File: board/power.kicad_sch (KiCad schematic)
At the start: 16 parts, among them J2 768250002, U2 OKI-78SR-12_1.0-W36H-C, U3 SHHD003A0A

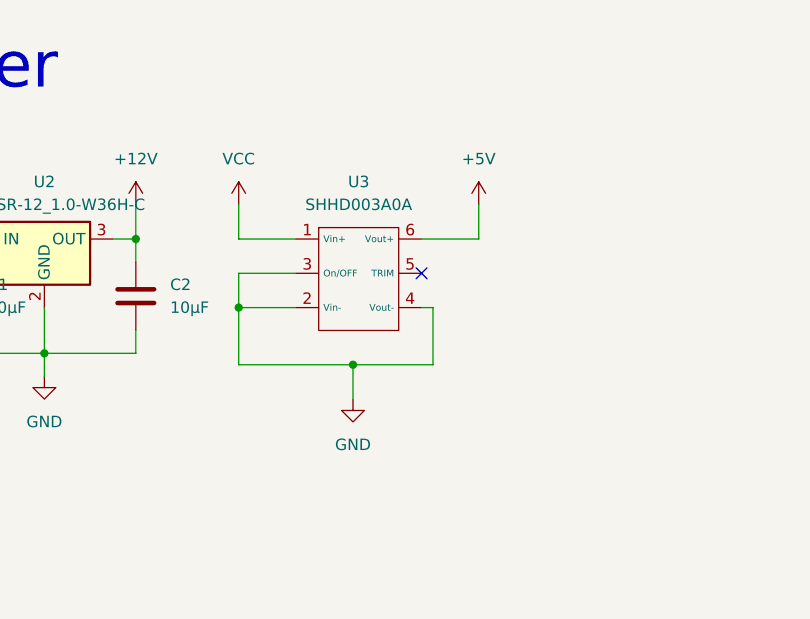
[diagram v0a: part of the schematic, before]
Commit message: rev2 progress
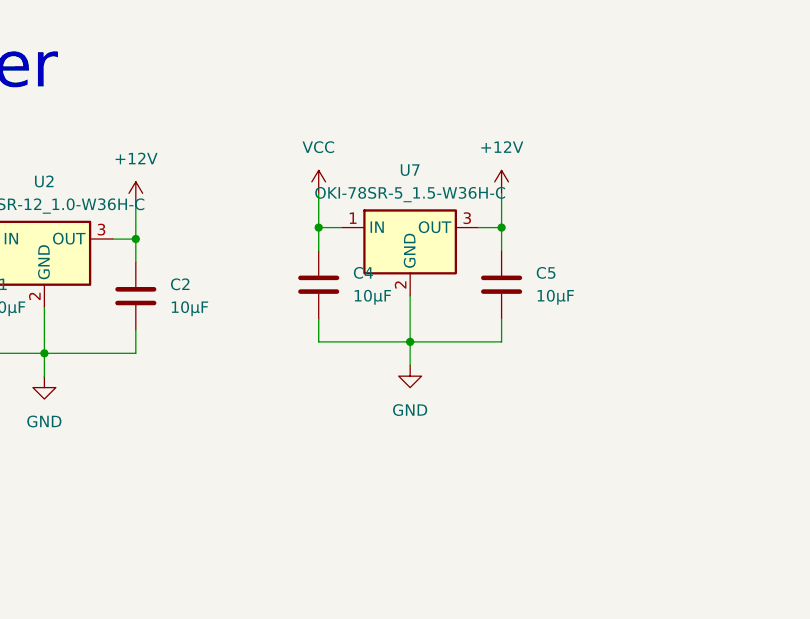
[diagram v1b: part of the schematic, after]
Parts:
- removed U3: SHHD003A0A, MRDT_Devices:SHHD003A0A-SRZ_Surface_Mount, symbol MRDT_Devices:SHHD003A0A
- added C4: 10µF, Capacitor_SMD:C_1206_3216Metric_Pad1.33x1.80mm_HandSolder, symbol Device:C
- added C5: 10µF, Capacitor_SMD:C_0603_1608Metric_Pad1.08x0.95mm_HandSolder, symbol Device:C
- added U7: OKI-78SR-5_1.5-W36H-C, Converter_DCDC:Converter_DCDC_Murata_OKI-78SR_Horizontal, symbol Converter_DCDC:OKI-78SR-5_1.5-W36H-C
- MOSFET1: footprint MRDT_Devices:SOP-8_TOS-L -> CoreBoard:MSOP8_MC_MCH-L
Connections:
- net +12V: now also C5.1, U7.3 (OUT)
- net GND: now also C4.2, C5.2, U7.2 (GND)
- net VCC: now also C4.1, U7.1 (IN)
- no-connect marks 1 -> 0
